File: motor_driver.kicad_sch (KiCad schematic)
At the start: 4 parts, among them M1 Motor_DC, U1 DRV8210PDSGR

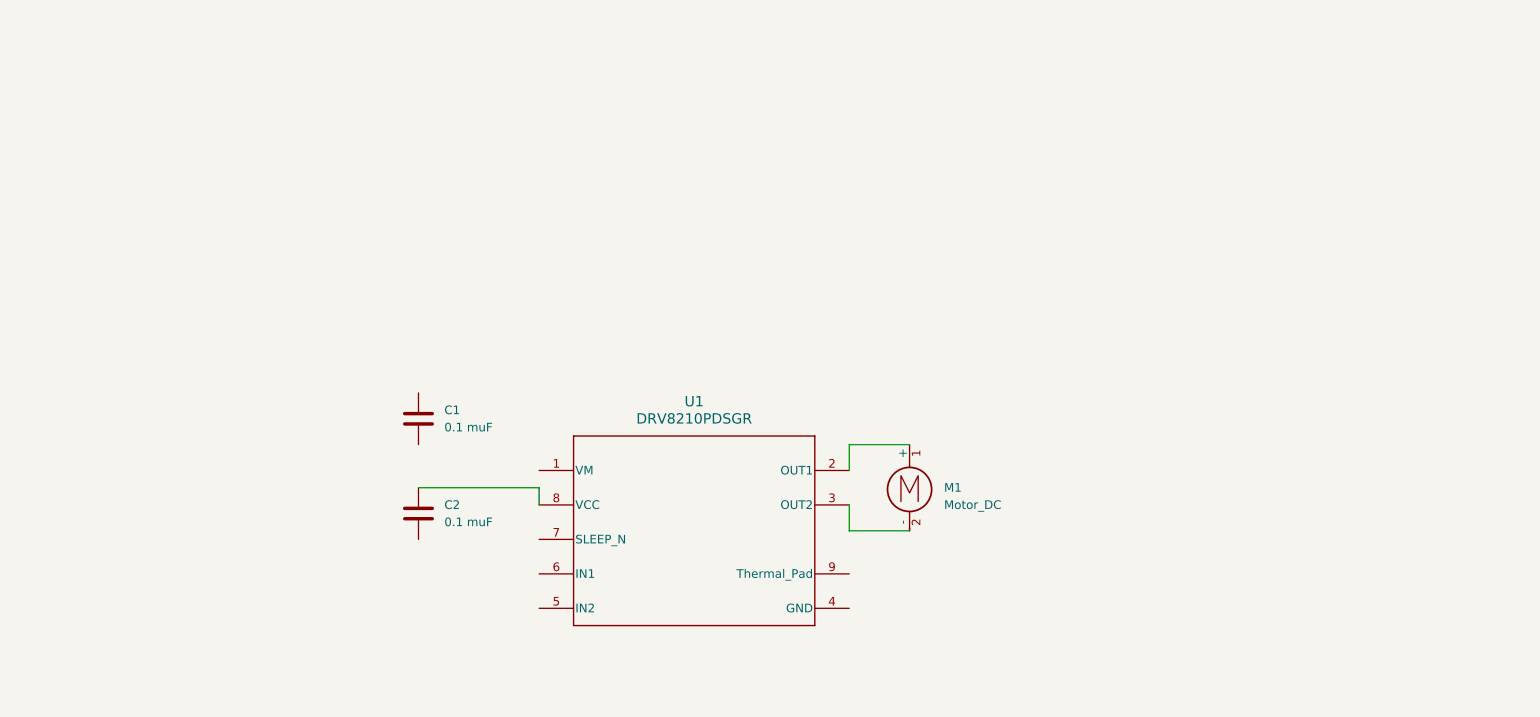
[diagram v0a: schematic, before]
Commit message: all the joy in life has disappeared
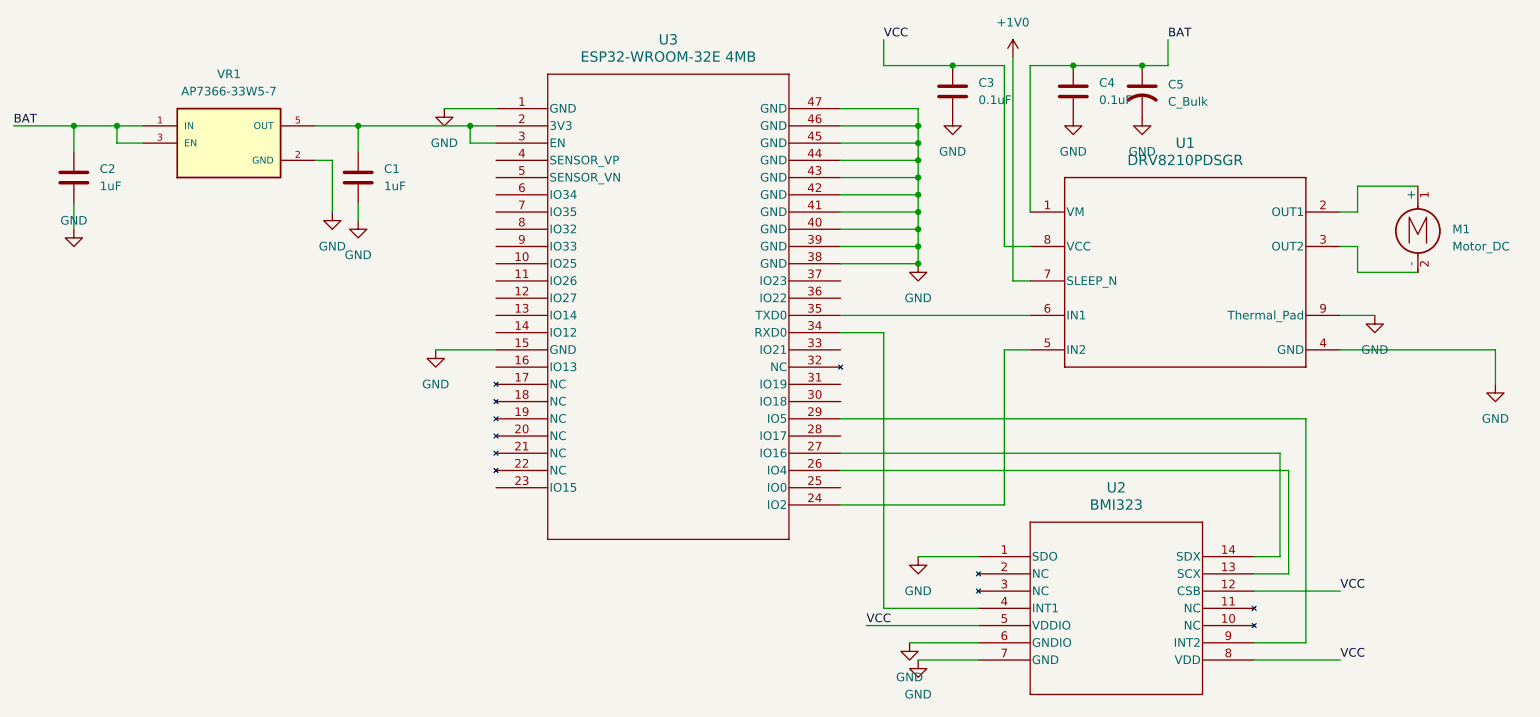
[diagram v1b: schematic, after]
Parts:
- added C3, C4: 0.1uF, symbol Device:C
- added C5: C_Bulk, symbol Device:C_US
- added U2: BMI323, BMI323_BOS, symbol BMI323:BMI323
- added U3: ESP32-WROOM-32E 4MB, symbol 2025-09-26_21-40-56:ESP32-WROOM-32E_4MB
- added VR1: AP7366-33W5-7, AP7366-33W5-7:SOT95P285X140-5N, symbol AP7366-33W5-7:AP7366-33W5-7
- C1, C2: value 0.1 muF -> 1uF
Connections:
- net at C1.1: now also U3.2 (3V3), U3.3 (EN), VR1.5 (OUT)
- net GND: now reaches C1.2
- net GND: now also C2.2, U1.4 (GND), U1.9 (Thermal_Pad), C3.2, C4.2, C5.2, U2.1 (SDO), U2.6 (GNDIO), U2.7 (GND), U3.1 (GND), U3.15 (GND), U3.38 (GND), U3.39 (GND), U3.40 (GND), U3.41 (GND), U3.42 (GND), U3.43 (GND), U3.44 (GND), U3.45 (GND), U3.46 (GND), U3.47 (GND), VR1.2 (GND)
- net BAT: now reaches U1.1 (VM)
- net BAT: now also C2.1, C4.1, C5.1, VR1.1 (IN), VR1.3 (EN)
- net at U1.5 (IN2): now also U3.24 (IO2)
- net at U1.6 (IN1): now also U3.35 (TXD0)
- net +1V0: now reaches U1.7 (SLEEP_N)
- net VCC: now reaches U1.8 (VCC)
- net VCC: now also C3.1, U2.12 (CSB), U2.5 (VDDIO), U2.8 (VDD); no longer C2.1
- new net: U2.13 (SCX), U3.26 (IO4)
- new net: U2.14 (SDX), U3.27 (IO16)
- new net: U2.4 (INT1), U3.34 (RXD0)
- new net: U2.9 (INT2), U3.29 (IO5)
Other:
- moved on the sheet: U1

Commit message: added footprints
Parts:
- U1: footprint DSG0008A-IPC_A -> DRV8210PDSGRfootprints:BMI323_BOS
- U2: footprint BMI323_BOS -> Bosch_IMU_footprints:BMI323_BOS
- U3: footprint (none) -> ESP32footprints:ESP32­WROOM­32E_EXP
- VR1: footprint AP7366-33W5-7:SOT95P285X140-5N -> AP7366_33W5_7:SOT95P285X140-5N
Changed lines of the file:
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@@
 			)
 		)
-		(property "Footprint" "BMI323_BOS"
+		(property "Footprint" "Bosch_IMU_footprints:BMI323_BOS"
 			(at 187.96 104.14 0)
 			(effects
@@
 			)
 		)
-		(property "Footprint" ""
+		(property "Footprint" "ESP32footprints:ESP32­WROOM­32E_EXP"
 			(at 142.24 64.77 0)
 			(effects
@@
 			)
 		)
-		(property "Footprint" "DSG0008A-IPC_A"
+		(property "Footprint" "DRV8210PDSGRfootprints:BMI323_BOS"
 			(at 195.58 53.34 0)
 			(effects
@@
 			)
 		)
-		(property "Footprint" "AP7366-33W5-7:SOT95P285X140-5N"
+		(property "Footprint" "AP7366_33W5_7:SOT95P285X140-5N"
 			(at 77.47 43.18 0)
 			(effects

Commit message: 4 motors :fearful:
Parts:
- C1, C2, C3, C4: footprint (none) -> Capacitor_SMD:C_0603_1608Metric
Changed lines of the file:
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@@
 			)
 		)
-		(property "Footprint" ""
+		(property "Footprint" "Capacitor_SMD:C_0603_1608Metric"
 			(at 185.1152 39.37 0)
 			(effects
@@
 			)
 		)
-		(property "Footprint" ""
+		(property "Footprint" "Capacitor_SMD:C_0603_1608Metric"
 			(at 202.8952 39.37 0)
 			(effects
@@
 			)
 		)
-		(property "Footprint" ""
+		(property "Footprint" "Capacitor_SMD:C_0603_1608Metric"
 			(at 55.5752 52.07 0)
 			(effects
@@
 			)
 		)
-		(property "Footprint" ""
+		(property "Footprint" "Capacitor_SMD:C_0603_1608Metric"
 			(at 97.4852 52.07 0)
 			(effects
